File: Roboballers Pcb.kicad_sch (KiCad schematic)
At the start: 116 parts, among them J1 Conn_01x02, J2 Conn_01x02, J3 Conn_01x02, J4 Conn_01x02, J5 Screw_Terminal_01x02, J6 Conn_01x02, J7 Bottom_Pcb, SW1 OS102011MS2QN1, SW2 OS102011MS2QN1, SW3 OS102011MS2QN1, SW4 OS102011MS2QN1, U1 VNH7070ASTR, U10 TSOP25xx, U11 OpenMV_H7_R2, U12 MCP3008, U13 TSOP25xx, U14 TSOP25xx, U15 SEN0140, U16 TSOP25xx, U17 RockerSwitch, U18 TSOP25xx, U19 TSOP25xx, U2 VNH7070ASTR, U20 TSOP25xx, U21 TSOP25xx, U22 TSOP25xx, U23 TSOP25xx, U24 TSOP25xx, U25 TSOP25xx, U26 TSOP25xx, U27 MCP3008, U28 MCP3008, U29 TSOP25xx, U3 VNH7070ASTR, U30 TSOP25xx, U31 TSOP25xx, U32 TSOP25xx, U33 TSOP25xx, U34 TSOP25xx, U35 TSOP25xx, U36 TSOP25xx, U4 VNH7070ASTR, U5 Teensy4.1, U6 TSOP25xx, U7 V_Regulator_-_5v, U8 TSOP25xx, U9 TSOP25xx

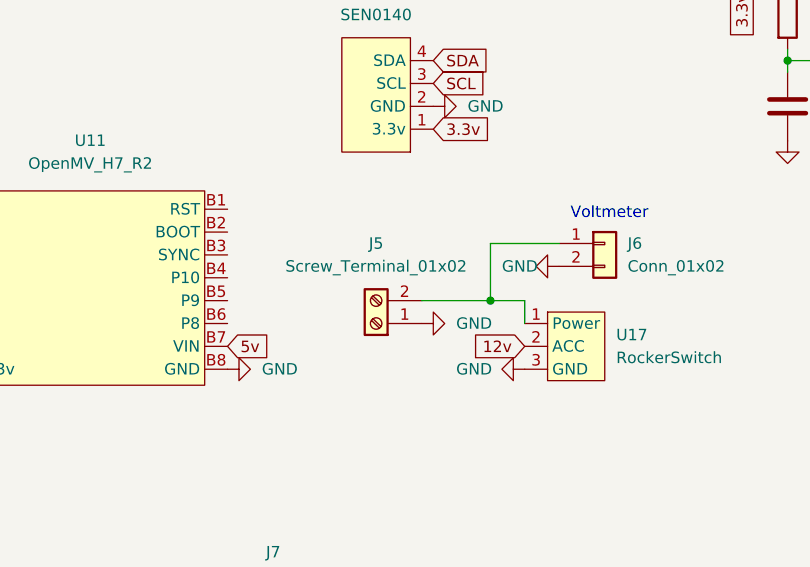
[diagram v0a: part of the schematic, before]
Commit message: should be done now!!
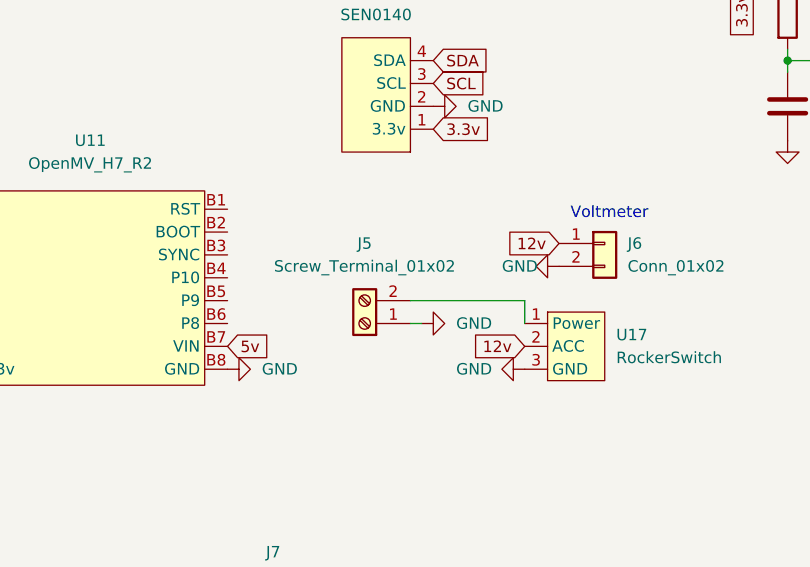
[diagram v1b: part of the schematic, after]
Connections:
- net 12v: now also J6.1 (Pin_1)
- net at J5.2 (Pin_2), U17.1 (Power): no longer J6.1 (Pin_1)
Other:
- moved on the sheet: J5
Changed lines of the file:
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@@
 	)
 	(junction
-		(at 238.76 199.39)
-		(diameter 0)
-		(color 0 0 0 0)
-	)
-	(junction
 		(at 100.33 54.61)
 		(diameter 0)
@@
 	(wire
 		(pts
+			(xy 229.87 201.93) (xy 231.14 201.93)
+		)
+		(stroke
+			(width 0)
+			(type default)
+		)
+	)
+	(wire
+		(pts
 			(xy 354.33 166.37) (xy 354.33 167.64)
 		)
@@
 	(wire
 		(pts
-			(xy 246.38 193.04) (xy 238.76 193.04)
-		)
-		(stroke
-			(width 0)
-			(type default)
-		)
-	)
-	(wire
-		(pts
 			(xy 326.39 107.95) (xy 331.47 107.95)
 		)
@@
 	(wire
 		(pts
-			(xy 238.76 199.39) (xy 242.57 199.39)
+			(xy 229.87 199.39) (xy 242.57 199.39)
 		)
 		(stroke
@@
 	(wire
 		(pts
-			(xy 238.76 193.04) (xy 238.76 199.39)
-		)
-		(stroke
-			(width 0)
-			(type default)
-		)
-	)
-	(wire
-		(pts
 			(xy 392.43 69.85) (xy 392.43 53.34)
 		)
@@
 	(wire
 		(pts
-			(xy 231.14 199.39) (xy 238.76 199.39)
-		)
-		(stroke
-			(width 0)
-			(type default)
-		)
-	)
-	(wire
-		(pts
 			(xy 91.44 123.19) (xy 100.33 123.19)
 		)
@@
 		)
 	)
+	(global_label "12v"
+		(shape input)
+		(at 246.38 193.04 180)
+		(fields_autoplaced yes)
+		(effects
+			(font
+				(size 1.27 1.27)
+			)
+			(justify right)
+		)
+		(property "Intersheetrefs" "${INTERSHEET_REFS}"
+			(at 240.0082 193.04 0)
+			(effects
+				(font
+					(size 1.27 1.27)
+				)
+				(justify right)
+				(hide yes)
+			)
+		)
+	)
 	(global_label "CLS1"
 		(shape input)
@@
 		)
 		(property "Intersheetrefs" "${INTERSHEET_REFS}"
-			(at 141.5202 200.7394 0)
+			(at 140.9482 200.66 0)
 			(effects
 				(font
@@
 		)
 		(property "Intersheetrefs" "${INTERSHEET_REFS}"
-			(at 236.7702 204.5494 0)
+			(at 236.1982 204.47 0)
 			(effects
 				(font
@@
 	(symbol
 		(lib_id "Connector:Screw_Terminal_01x02")
-		(at 226.06 201.93 180)
+		(at 224.79 201.93 180)
 		(unit 1)
 		(exclude_from_sim no)
@@
 		(fields_autoplaced yes)
 		(property "Reference" "J5"
-			(at 226.06 193.04 0)
+			(at 224.79 193.04 0)
 			(effects
 				(font
@@
 		)
 		(property "Value" "Screw_Terminal_01x02"
-			(at 226.06 195.58 0)
+			(at 224.79 195.58 0)
 			(effects
 				(font
@@
 		)
 		(property "Footprint" "Pads:Pads"
-			(at 226.06 201.93 0)
+			(at 224.79 201.93 0)
 			(effects
 				(font
@@
 		)
 		(property "Datasheet" "~"
-			(at 226.06 201.93 0)
+			(at 224.79 201.93 0)
 			(effects
 				(font
@@
 		)
 		(property "Description" ""
-			(at 226.06 201.93 0)
+			(at 224.79 201.93 0)
 			(effects
 				(font
